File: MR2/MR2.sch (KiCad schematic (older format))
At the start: 12 parts, among them J1 Conn_01x04_Male, J2 Conn_01x04_Male, J3 Conn_01x04_Male, J4 Conn_01x04_Male, J5 Conn_01x02_Male, J6 Conn_01x02_Male, J7 Conn_01x04_Male, J8 Conn_01x02_Male, J9 Conn_01x02_Male, U5 LPC1768, U8 MCP2561-E-P

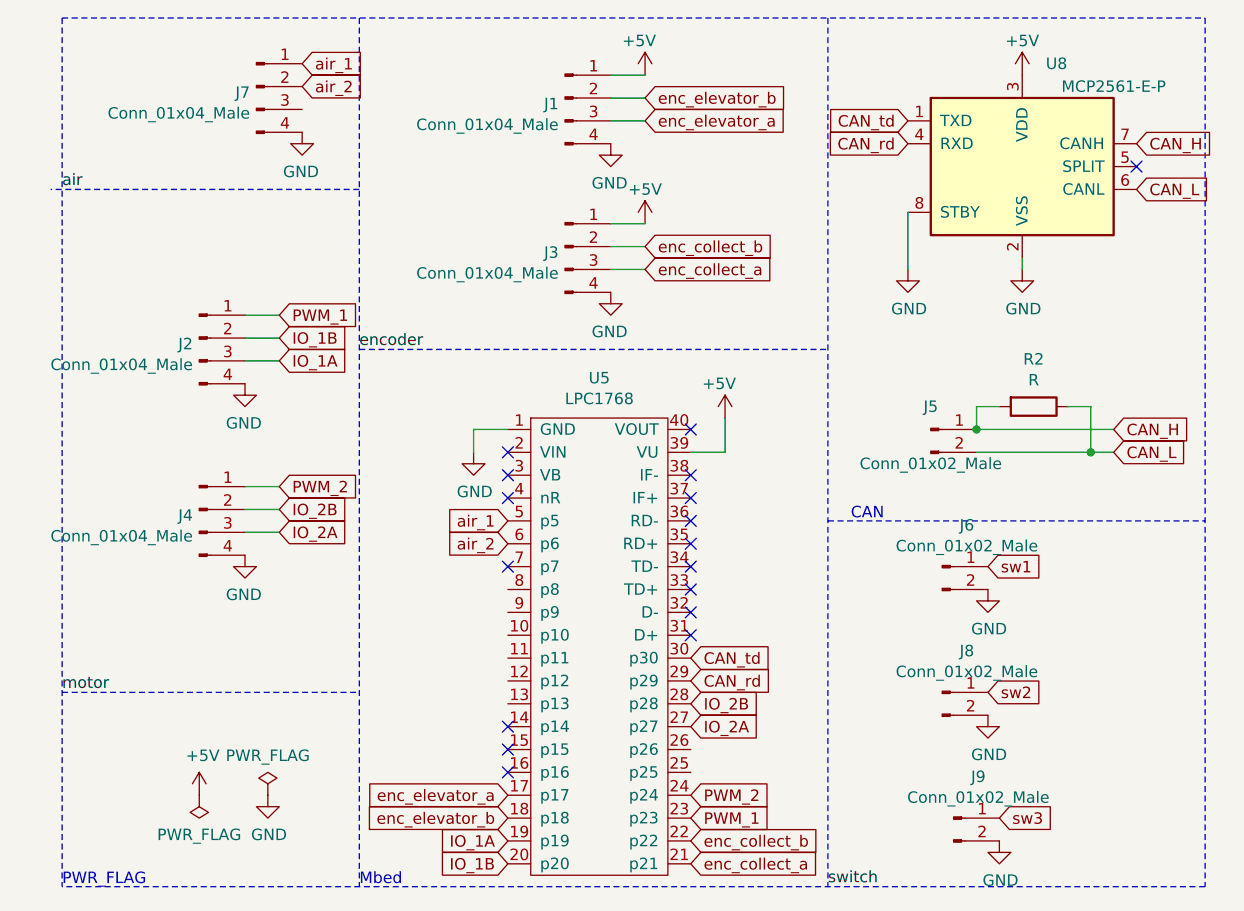
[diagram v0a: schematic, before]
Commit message: update:MR2の基板完成
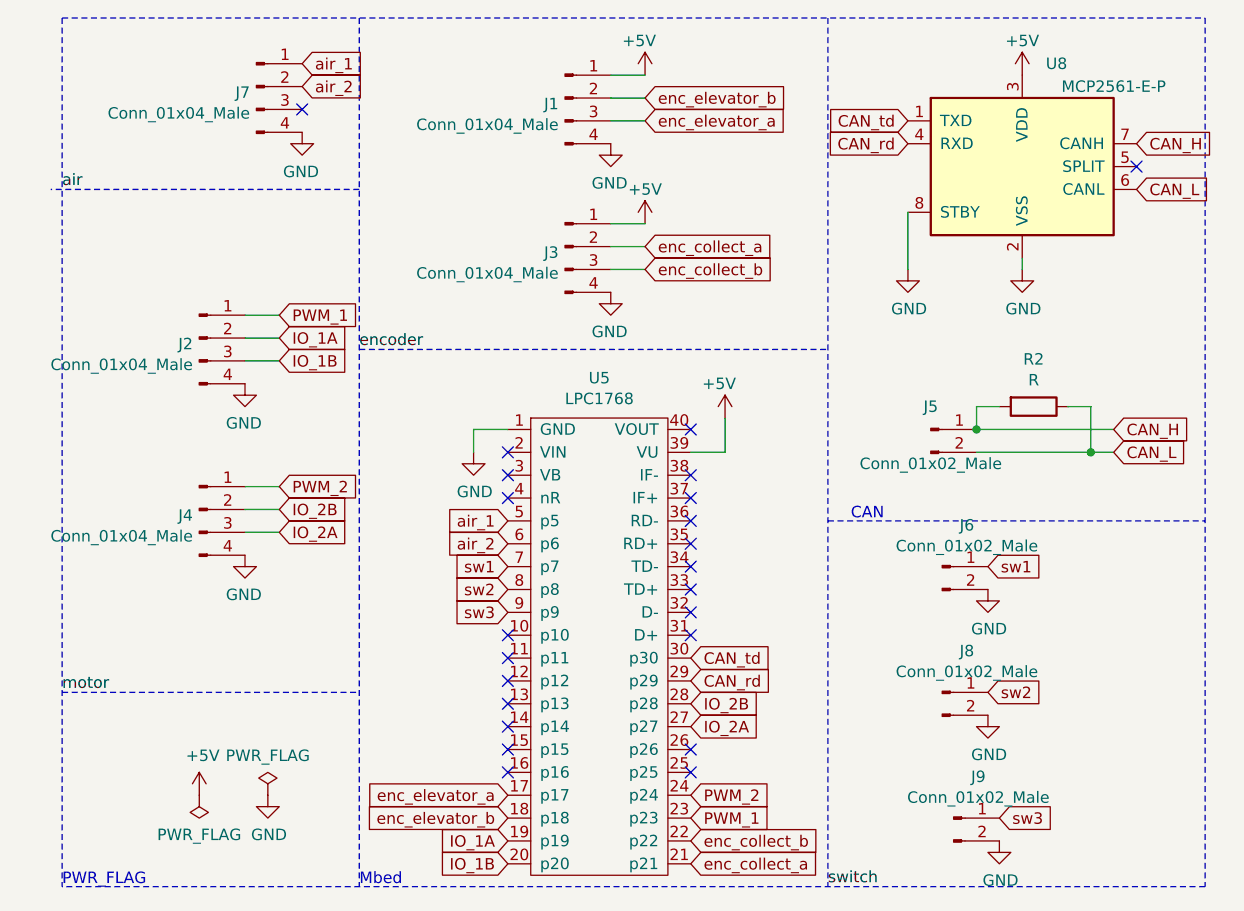
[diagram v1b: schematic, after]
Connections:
- net IO_1A: now also J2.2 (Pin_2); no longer J2.3 (Pin_3)
- net IO_1B: now also J2.3 (Pin_3); no longer J2.2 (Pin_2)
- net enc_collect_a: now also J3.2 (Pin_2); no longer J3.3 (Pin_3)
- net enc_collect_b: now also J3.3 (Pin_3); no longer J3.2 (Pin_2)
- net sw1: now also U5.7 (p7)
- net sw2: now also U5.8 (p8)
- net sw3: now also U5.9 (p9)
- no-connect marks 17 -> 23
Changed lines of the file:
@@
 Text GLabel 4300 3200 2    50   Input ~ 0
 PWM_1
+Text GLabel 4300 3400 2    50   Input ~ 0
+IO_1B
 Text GLabel 4300 3300 2    50   Input ~ 0
-IO_1B
-Text GLabel 4300 3400 2    50   Input ~ 0
 IO_1A
 Wire Wire Line
@@
 Text GLabel 5900 2350 2    50   Input ~ 0
 enc_elevator_a
+Text GLabel 5900 3000 2    50   Input ~ 0
+enc_collect_b
 Text GLabel 5900 2900 2    50   Input ~ 0
-enc_collect_b
-Text GLabel 5900 3000 2    50   Input ~ 0
 enc_collect_a
 Wire Notes Line
@@
 	1    0    0    -1
 $EndComp
-NoConn ~ 5300 4300
 Text Label 3350 4850 0    50   ~ 0
 motor
 Text Label 6700 5700 0    50   ~ 0
 switch
+NoConn ~ 5300 4600
+NoConn ~ 5300 4700
+NoConn ~ 5300 4800
+NoConn ~ 5300 4900
+NoConn ~ 6100 5100
+NoConn ~ 6100 5200
+NoConn ~ 4400 2300
+Text GLabel 5300 4300 0    50   Input ~ 0
+sw1
+Text GLabel 5300 4400 0    50   Input ~ 0
+sw2
+Text GLabel 5300 4500 0    50   Input ~ 0
+sw3
 $EndSCHEMATC
